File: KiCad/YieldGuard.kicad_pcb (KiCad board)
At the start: 2 copper layers, 55 x 60 mm, 4 parts, among them J1 Conn_01x04_Socket, U1 ESP32-DEVKITC, U2 HX711

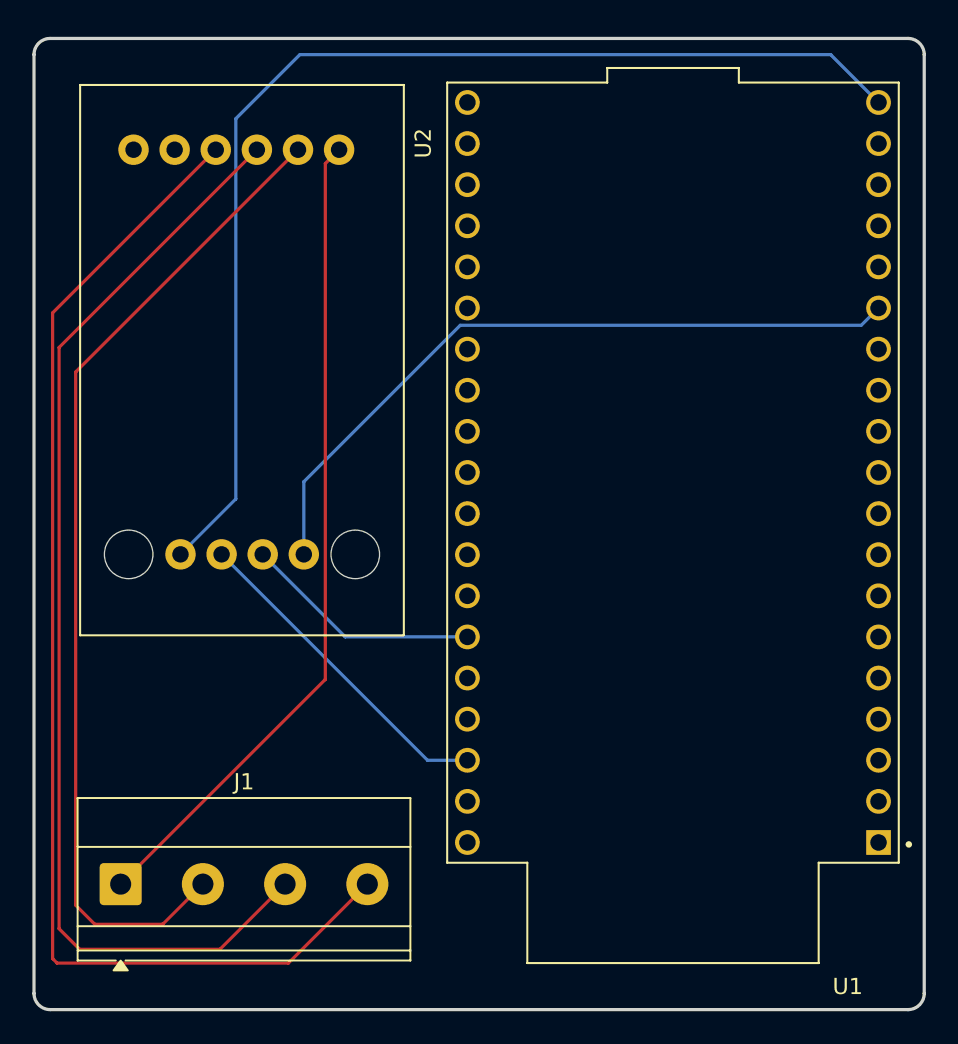
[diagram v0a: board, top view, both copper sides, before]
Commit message: Bit changes in PCB and Schematic and Completed BoM
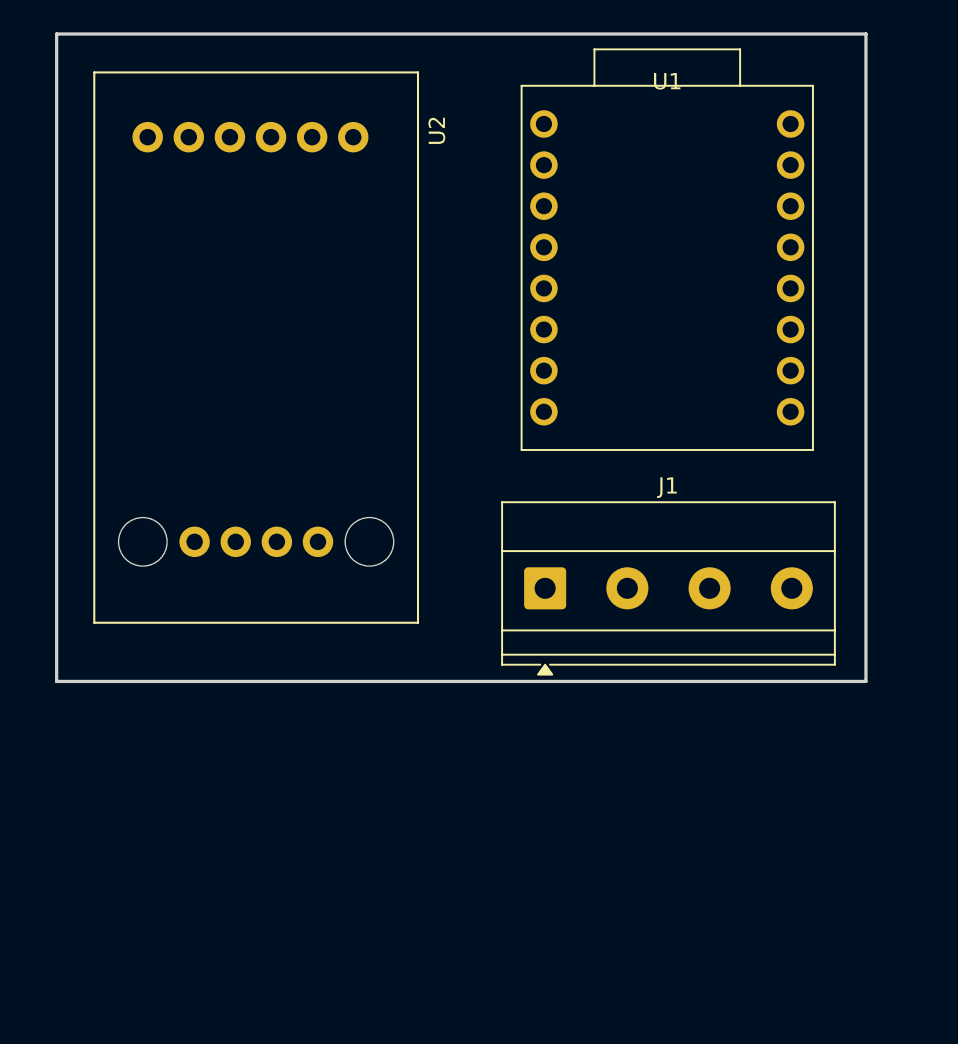
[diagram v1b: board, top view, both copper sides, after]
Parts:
- U1: value ESP32-DEVKITC -> ESP32_C3_Super_Mini; footprint KiCad:MODULE_ESP32-DEVKITC -> KiCad:ESP32-C3_SuperMini
- moved J1 32.0 mm to (136.2, 73.4)
- moved G*** 26.9 mm to (114.3, 56.4)
- moved U1 12.7 mm to (143.7, 53.6), turned to 0 degrees
- moved U2 1.17 mm to (118.3, 58.5)
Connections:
- U1 pad 1: unconnected-(U1-3V3-Pad1) -> /5V
- U1 pad 14: /GND -> unconnected-(U1-GPIO10-Pad14)
- U1 pad 2: unconnected-(U1-EN-Pad2) -> /GND
- U1 pad 4: unconnected-(U1-SENSOR_VN-Pad4) -> /DATA
- U1 pad 9: unconnected-(U1-IO25-Pad9) -> /CLOCK
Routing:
- net /GREEN_WIRE: track 75.7 -> 0.00 mm
- net /5V: track 70.9 -> 0.00 mm
- net /WHITE_WIRE: track 69.3 -> 0.00 mm
- net /BLACK_WIRE_GND: track 61.7 -> 0.00 mm
- net /RED_WIRE_PWR: track 51.0 -> 0.00 mm
- net /GND: track 44.4 -> 0.00 mm
- net /CLOCK: track 20.5 -> 0.00 mm
- net /DATA: track 14.8 -> 0.00 mm
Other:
- board size 55 x 60 mm -> 50 x 40 mm
- board text removed: "Designed by Safeer Hassan :)"
